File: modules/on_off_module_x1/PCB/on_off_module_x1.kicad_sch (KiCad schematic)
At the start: 31 parts, among them J1 Screw_Terminal_01x02, J2 Screw_Terminal_01x02, J3 Screw_Terminal_01x02, J4 Conn_01x06_Socket, J5 Conn_01x03_Socket, K1 12V 5A, Q1 2N7002H, SW1 SW_SPDT, U1 AMS1117-3.3, U2 ESP-12E, U3 PC817, U4 H11AA1

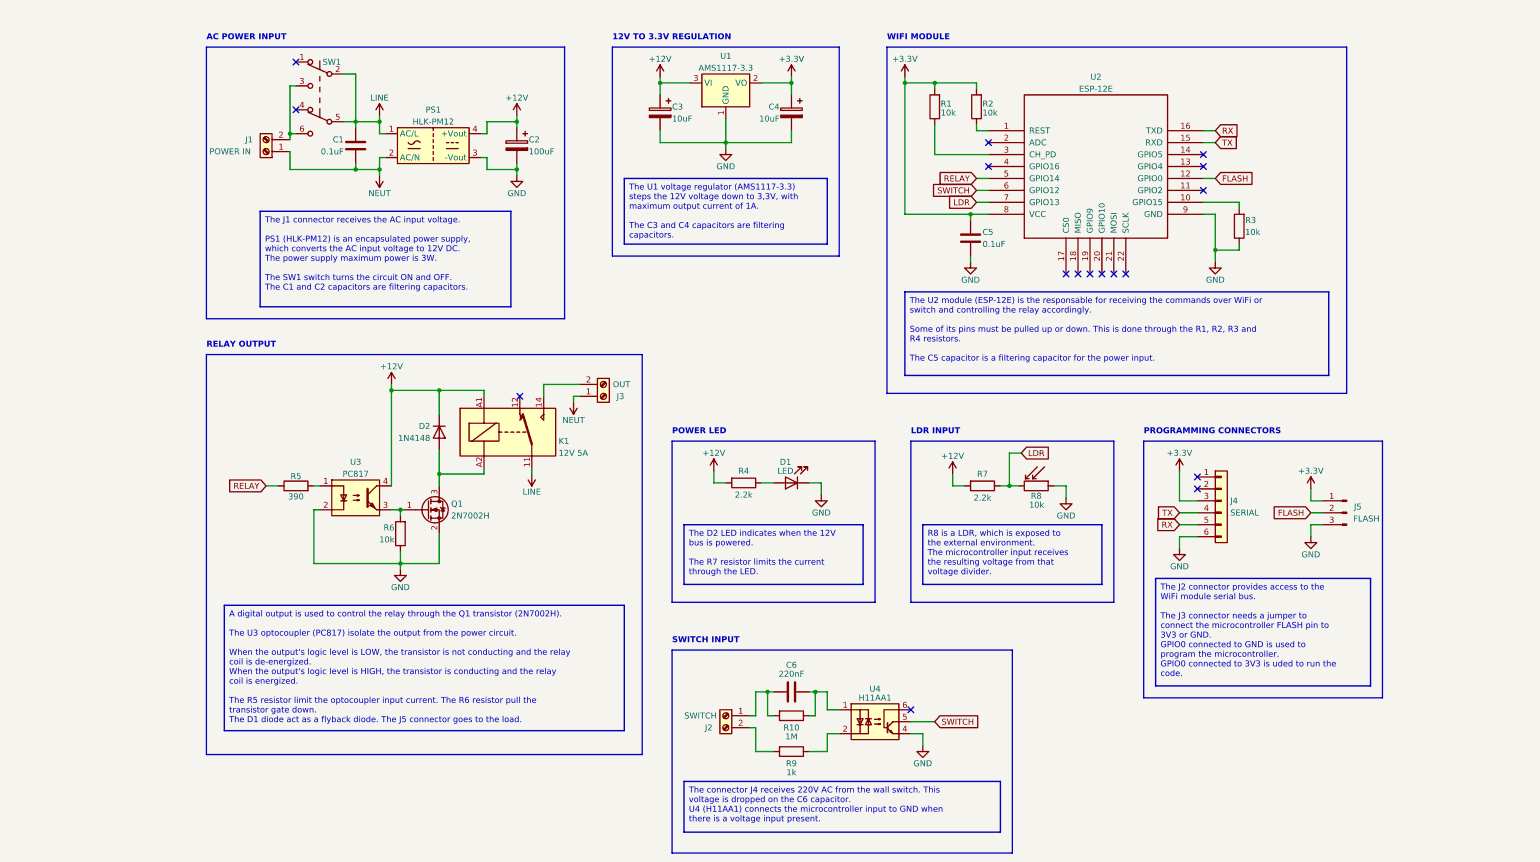
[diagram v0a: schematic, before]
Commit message: General files structure refactoring
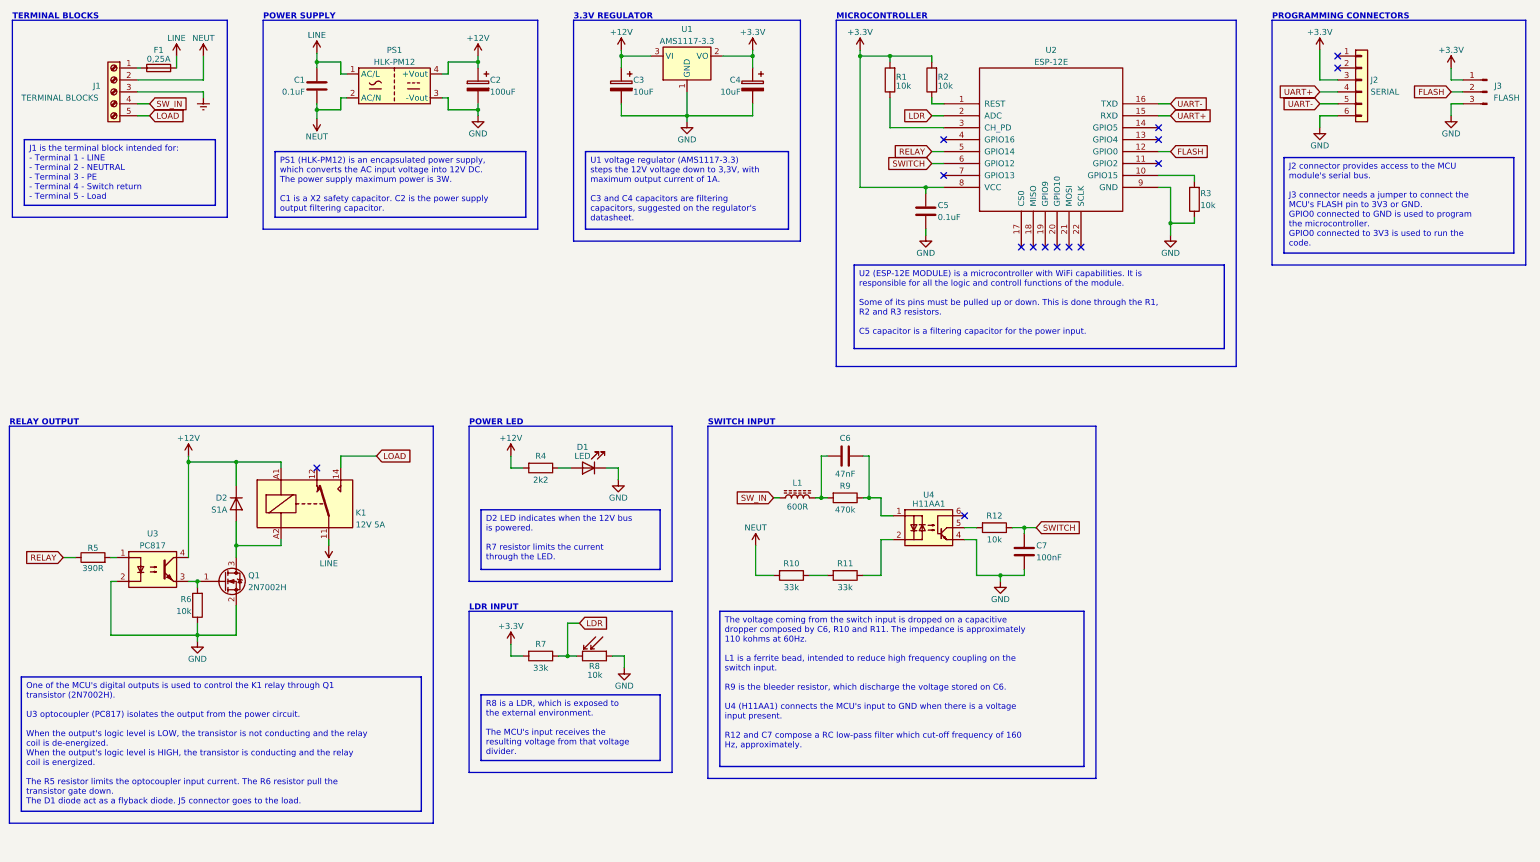
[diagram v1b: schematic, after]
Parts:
- removed D2: 1N4148, Alan_Diode:DIODE_SMD_SOD323F, symbol Alan_Diode:DIODE_1N4148
- removed J1, J2, J3: Screw_Terminal_01x02, Alan_Connector:CONN_TERMINAL-BLOCK_2P_P5.08, symbol Alan_Connector:CONN_TERMINAL-BLOCK_2P_P5.08
- removed SW1: SW_SPDT, Alan_Switches:SW_TOGGLE_DPDT_THT_7x7, symbol Alan_Switches:SW_TOGGLE_DPDT_THT_7x7
- added C7: 100nF, Alan_Capacitor:CAP_SMD_CERAMIC_0603, symbol Alan_Capacitor:CAP_SMD_CERAMIC_0603
- added D2: S1A, Alan_Diode:DIODE_SMD_SMA, symbol Alan_Diode:DIODE_S1A
- added F1: 0,25A, Alan_Fuse:FUSEHOLDER_THT_5x20_CLIP, symbol Alan_Fuse:FUSEHOLDER_THT_5x20_CLIP
- added J1: CONN_TERMINAL-BLOCK_5P_P5.08, Alan_Connector:CONN_TERMINAL-BLOCK_5P_P5.08, symbol Alan_Connector:CONN_TERMINAL-BLOCK_5P_P5.08
- added L1: 600R, Alan_Inductor:BEAD_SMD_1206, symbol Alan_Inductor:BEAD_SMD_1206
- added R11: 33k, Alan_Resistor:RES_SMD_1206, symbol Alan_Resistor:RES_SMD_1206
- added R12: 10k, Alan_Resistor:RES_SMD_0603, symbol Alan_Resistor:RES_SMD_0603
- C6: value 220nF -> 47nF; footprint Alan_Capacitor:CAP_THT_CERAMIC_X2_13x6x12 -> Alan_Capacitor:CAP_THT_CERAMIC_X2_13x5x11_P10; symbol Alan_Capacitor:CAP_THT_CERAMIC_X2_13x6x12 -> Alan_Capacitor:CAP_THT_CERAMIC_X2_13x5x11_P10; Voltage (none) -> 350V
- R10: value 1M -> 33k; Power (none) -> 1/4W; Tolerance (none) -> 5%
- R4: value 2.2k -> 2k2
- R5: value 390 -> 390R
- R7: value 2.2k -> 33k
- R9: value 1k -> 470k; Power (none) -> 1/4; Tolerance (none) -> 5%
- renumbered J4 to J2, J5 to J3
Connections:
- net +12V: now also D2.1 (K); no longer R7.1
- net +3.3V: now also R7.1
- net GND: now also C7.2
- net LDR: now also U2.2 (ADC); no longer U2.7 (GPIO13)
- net LINE: now also F1.2
- net NEUT: now also R10.1, J1.2 (Pin_2)
- net SWITCH: now also C7.1, R12.2; no longer U4.5
- net at C6.1: now also R9.1, L1.2; no longer R10.1
- net at C6.2, U4.1: now also R9.2; no longer R10.2
- net LOAD: now reaches K1.14
- net LOAD: now also J1.5 (Pin_5)
- net at K1.A2, Q1.3 (D): now also D2.2 (A)
- net at U4.2: now also R11.2; no longer R9.2
- net RX renamed UART-
- net TX renamed UART+
- new net: F1.1, J1.1 (Pin_1)
- new net: R12.1, U4.5
- new net: R10.2, R11.1
- new net Earth: J1.3 (Pin_3)
- new net SW_IN: J1.4 (Pin_4), L1.1
- no-connect marks 17 -> 15
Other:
- note added: "3.3V REGULATOR"
- note added: "MICROCONTROLLER"
- note added: "POWER SUPPLY"
- note added: "TERMINAL BLOCKS"
- note removed: "12V TO 3.3V REGULATION"
- note removed: "AC POWER INPUT"
- note removed: "WIFI MODULE"
- moved on the sheet: C1, C2, C3, C4, C5, C6, D1, J2, J3, K1, PS1, Q1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
